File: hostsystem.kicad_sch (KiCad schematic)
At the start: 79 parts, among them J1001 TC2050, J1002 Conn_01x03_Pin, U1001 AM6231ASGGGAALW, U1002 SN74LVC2G241DCUR, U1003 AT24C32D-STUM-T, X1001 32.768kHz, X1002 25MHz

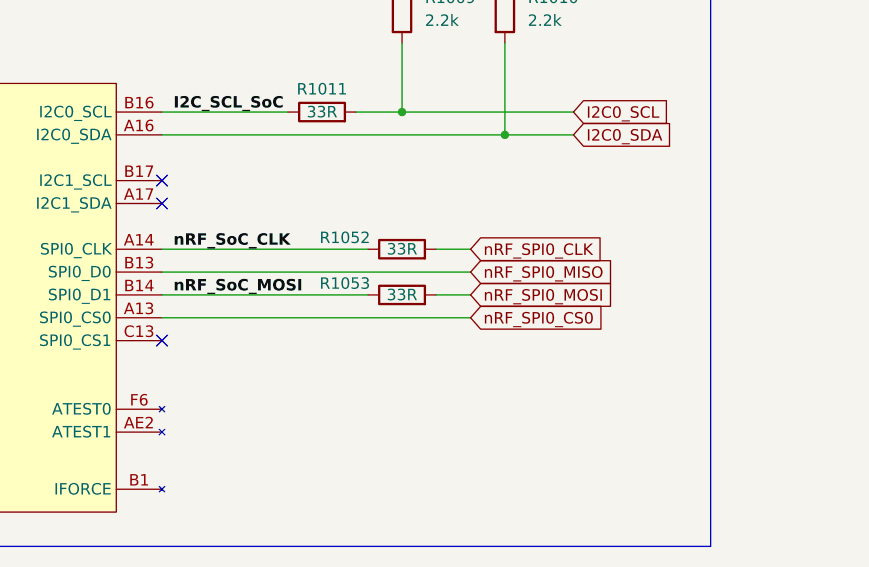
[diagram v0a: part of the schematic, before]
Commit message: Small fixes
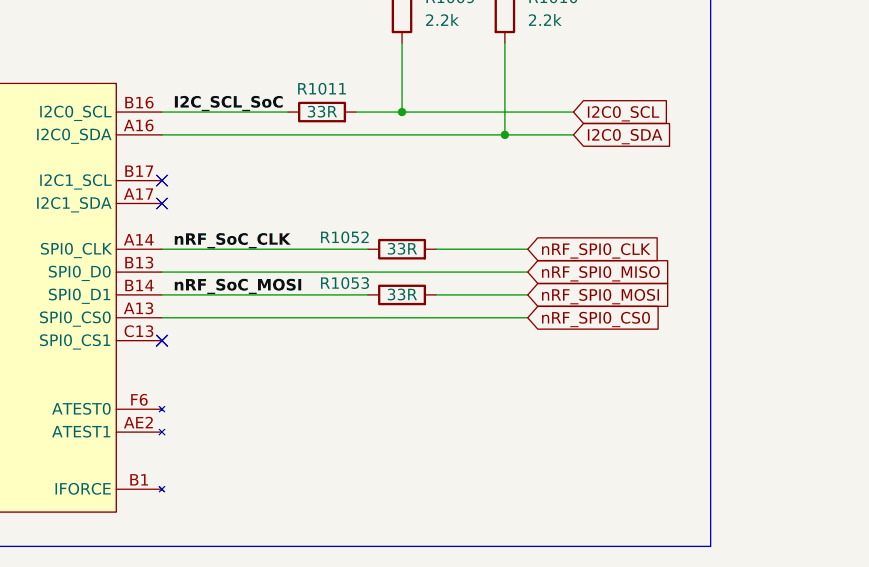
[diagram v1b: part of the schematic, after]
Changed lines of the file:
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@@
 	(wire
 		(pts
-			(xy 393.7 193.04) (xy 397.51 193.04)
+			(xy 393.7 193.04) (xy 403.86 193.04)
 		)
 		(stroke
@@
 	(wire
 		(pts
-			(xy 393.7 198.12) (xy 397.51 198.12)
+			(xy 393.7 198.12) (xy 403.86 198.12)
 		)
 		(stroke
@@
 	(wire
 		(pts
-			(xy 363.22 195.58) (xy 397.51 195.58)
+			(xy 363.22 195.58) (xy 403.86 195.58)
 		)
 		(stroke
@@
 	(wire
 		(pts
-			(xy 363.22 200.66) (xy 397.51 200.66)
+			(xy 363.22 200.66) (xy 403.86 200.66)
 		)
 		(stroke
@@
 	(global_label "nRF_SPI0_MISO"
 		(shape input)
-		(at 397.51 195.58 0)
+		(at 403.86 195.58 0)
 		(fields_autoplaced yes)
 		(effects
@@
 		)
 		(property "Intersheetrefs" "${INTERSHEET_REFS}"
-			(at 414.828 195.58 0)
+			(at 421.178 195.58 0)
 			(effects
 				(font
@@
 	(global_label "nRF_SPI0_CLK"
 		(shape input)
-		(at 397.51 193.04 0)
+		(at 403.86 193.04 0)
 		(fields_autoplaced yes)
 		(effects
@@
 		)
 		(property "Intersheetrefs" "${INTERSHEET_REFS}"
-			(at 413.7999 193.04 0)
+			(at 420.1499 193.04 0)
 			(effects
 				(font
@@
 	(global_label "nRF_SPI0_MOSI"
 		(shape input)
-		(at 397.51 198.12 0)
+		(at 403.86 198.12 0)
 		(fields_autoplaced yes)
 		(effects
@@
 		)
 		(property "Intersheetrefs" "${INTERSHEET_REFS}"
-			(at 414.828 198.12 0)
+			(at 421.178 198.12 0)
 			(effects
 				(font
@@
 	(global_label "nRF_SPI0_CS0"
 		(shape input)
-		(at 397.51 200.66 0)
+		(at 403.86 200.66 0)
 		(fields_autoplaced yes)
 		(effects
@@
 		)
 		(property "Intersheetrefs" "${INTERSHEET_REFS}"
-			(at 413.9208 200.66 0)
+			(at 420.2708 200.66 0)
 			(effects
 				(font
